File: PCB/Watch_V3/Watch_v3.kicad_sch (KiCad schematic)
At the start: 29 parts, among them J1 USB_C_Receptacle_USB2.0_16P, Q1 AO3401A, SW1 SW_DPST_x2, U1 AP2112K-3.3, U2 AP2112K-3.3, U3 AP2112K-3.3, U4 AP2112K-3.3

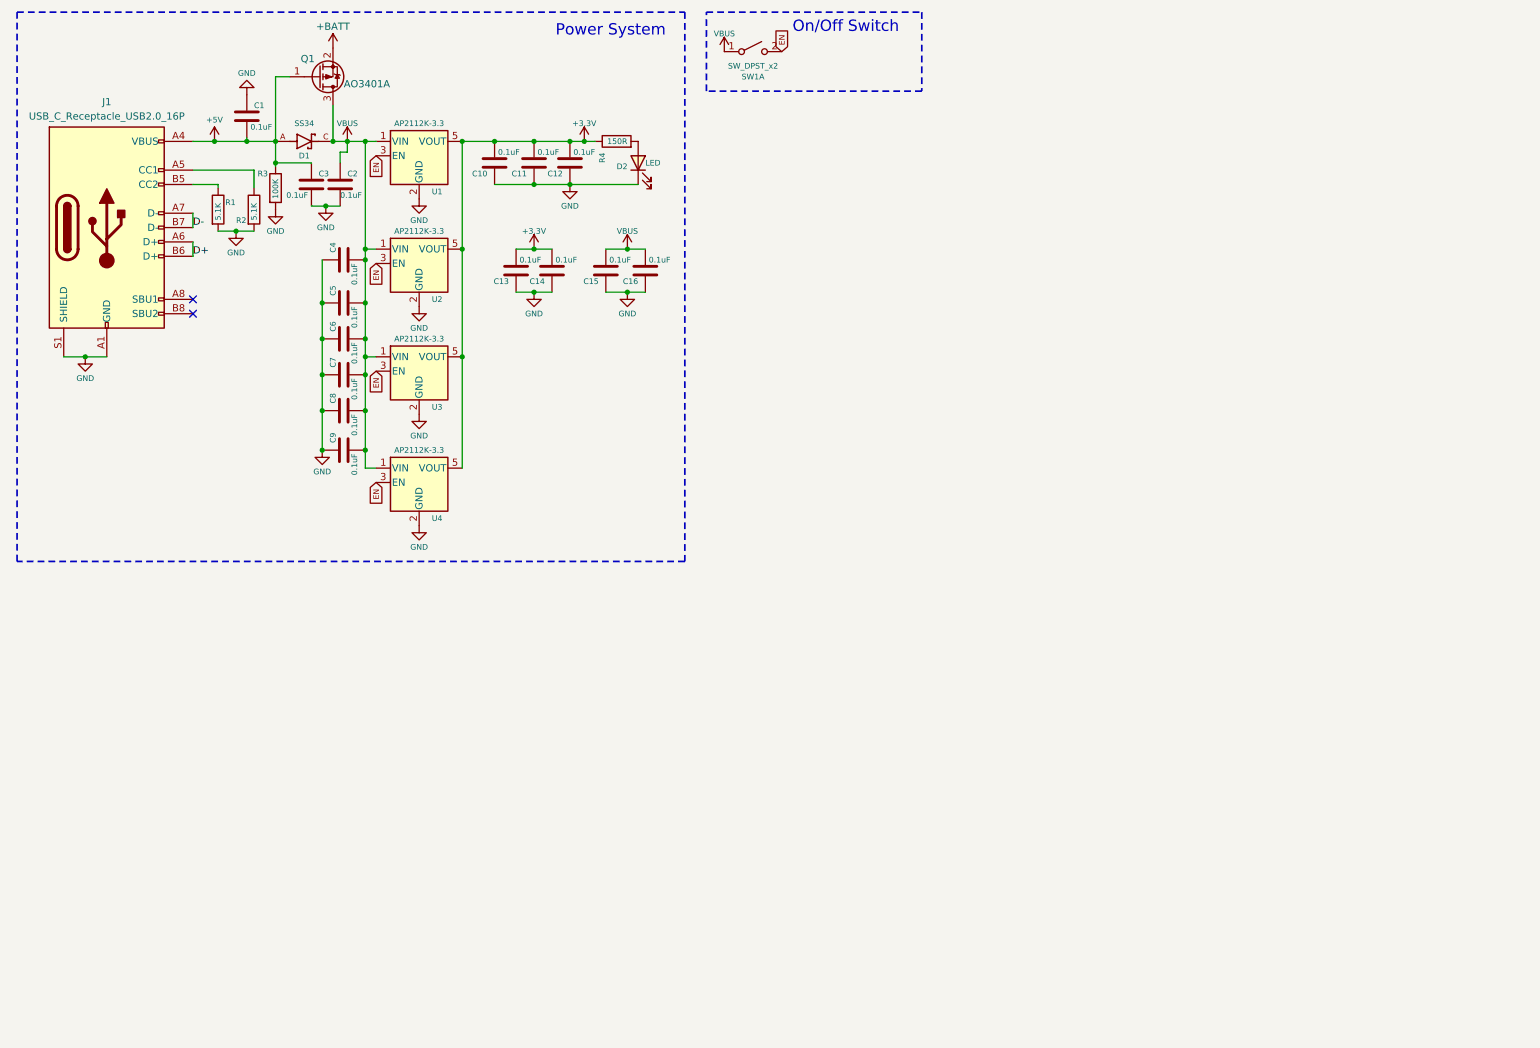
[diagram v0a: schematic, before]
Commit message: update PCB_watchV3
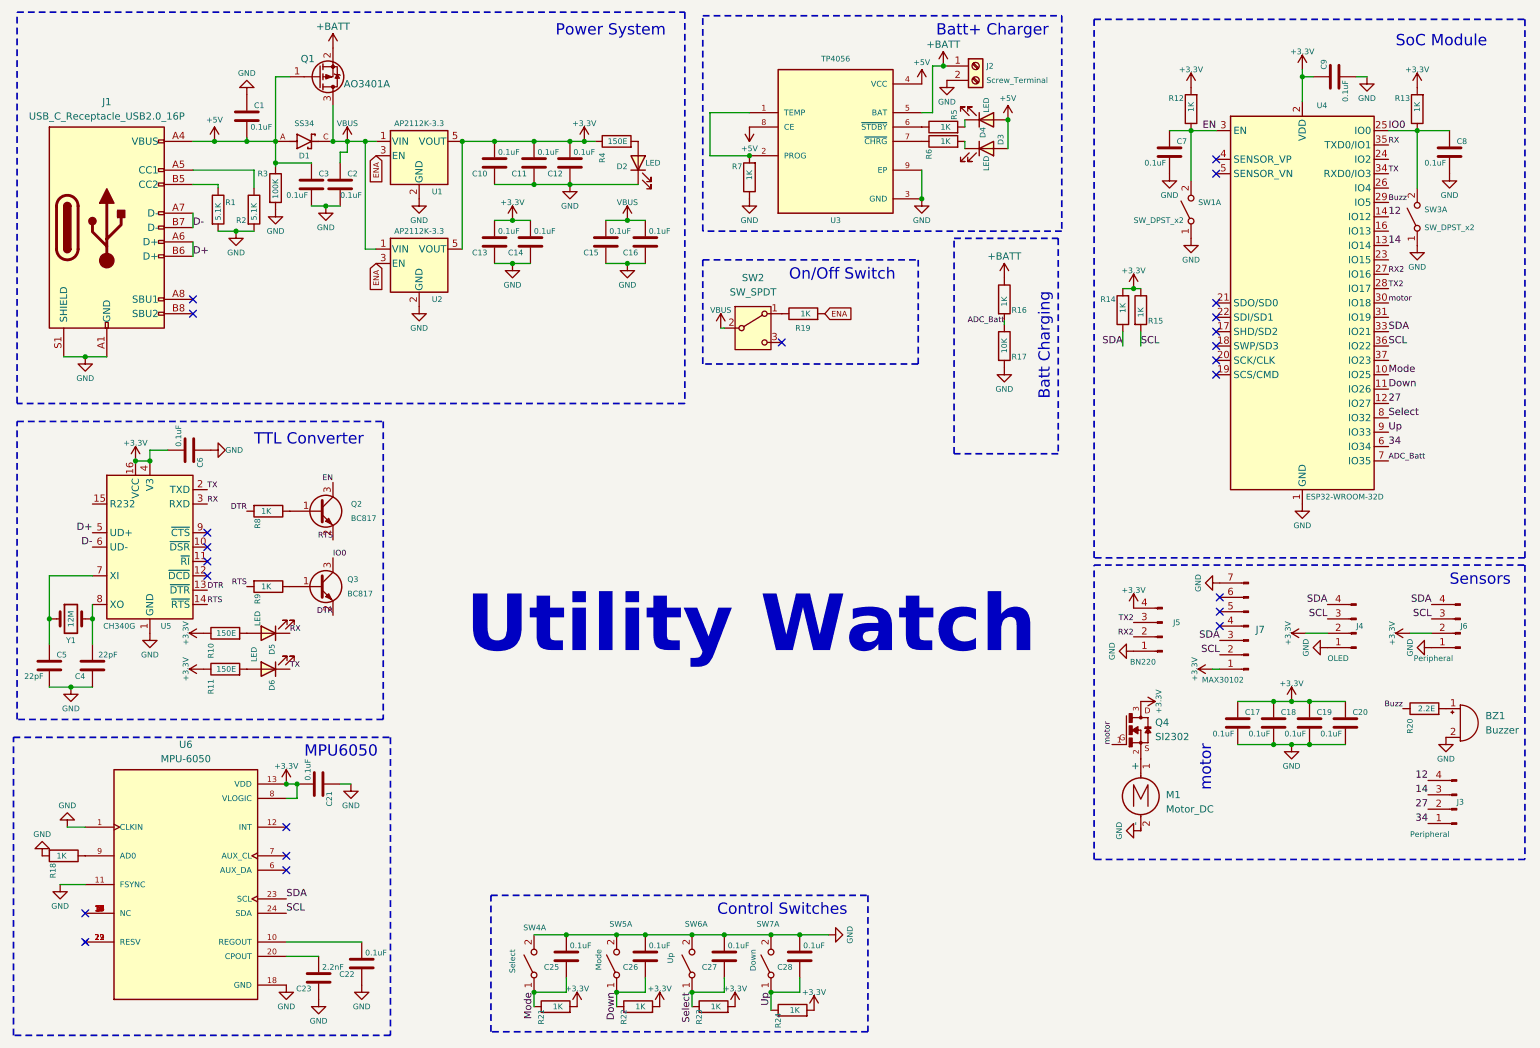
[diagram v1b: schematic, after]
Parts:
- removed U3, U4: AP2112K-3.3, Package_TO_SOT_SMD:SOT-23-5, symbol Regulator_Linear:AP2112K-3.3
- added BZ1: Buzzer, Buzzer_Beeper:Buzzer_12x9.5RM7.6, symbol Device:Buzzer
- added C17, C18, C19, C20, C21, C22, C25, C26, C27, C28: 0.1uF, Capacitor_SMD:C_0402_1005Metric, symbol Device:C
- added C23: 2.2nF, Capacitor_SMD:C_0402_1005Metric, symbol Device:C
- added D3, D4, D5, D6: LED, LED_SMD:LED_0402_1005Metric, symbol Device:LED
- added J2: Screw_Terminal, Button_Switch_SMD:solder_pad_batt, symbol Connector:Screw_Terminal_01x02
- added J3, J6: Peripheral, Button_Switch_SMD:solder_pad_4, symbol Connector:Conn_01x04_Pin
- added J4: OLED, Connector_PinHeader_2.54mm:PinHeader_1x04_P2.54mm_Vertical, symbol Connector:Conn_01x04_Pin
- added J5: BN220, Button_Switch_SMD:solder_pad_4, symbol Connector:Conn_01x04_Pin
- added J7: MAX30102, Connector_PinHeader_2.54mm:PinHeader_1x07_P2.54mm_Vertical, symbol Connector:Conn_01x07_Pin
- added M1: Motor_DC, Button_Switch_SMD:solder_motor, symbol Motor:Motor_DC
- added Q2, Q3: BC817, Package_TO_SOT_SMD:SOT-23, symbol Transistor_BJT:BC817
- added Q4: SI2302, SI2302:SOT23, symbol SI2302:SI2302
- added R10, R11: 150E, Resistor_SMD:R_01005_0402Metric, symbol Device:R
- added R12, R13, R14, R15, R16, R18, R19, R21, R22, R23, R24, R5, R6, R7, R8, R9: 1K, Resistor_SMD:R_01005_0402Metric, symbol Device:R
- added R17: 10K, Resistor_SMD:R_01005_0402Metric, symbol Device:R
- added R20: 2.2E, Resistor_SMD:R_01005_0402Metric, symbol Device:R
- added SW2: SW_SPDT, Button_Switch_THT:SW_Slide_1P2T_CK_OS102011MS2Q, symbol Switch:SW_SPDT
- added SW3: SW_DPST_x2, Button_Switch_SMD:SW_Push_1P1T_NO_6x6mm_H9.5mm, symbol Switch:SW_DPST_x2
- added SW4: Select, Button_Switch_SMD:SW_Push_1P1T_NO_6x6mm_H9.5mm, symbol Switch:SW_DPST_x2
- added SW5: Mode, Button_Switch_SMD:SW_Push_1P1T_NO_6x6mm_H9.5mm, symbol Switch:SW_DPST_x2
- added SW6: Up, Button_Switch_SMD:SW_Push_1P1T_NO_6x6mm_H9.5mm, symbol Switch:SW_DPST_x2
- added SW7: Down, Button_Switch_SMD:SW_Push_1P1T_NO_6x6mm_H9.5mm, symbol Switch:SW_DPST_x2
- added U3: TP4056, TP4056:SOP127P600X175-9N, symbol Amplifier_Audio:TP4056
- added U4: ESP32-WROOM-32D, RF_Module:ESP32-WROOM-32D, symbol RF_Module:ESP32-WROOM-32D
- added U5: CH340G, Package_SO:SOIC-16_3.9x9.9mm_P1.27mm, symbol Interface_USB:CH340G
- added U6: MPU-6050, Button_Switch_SMD:QFN50P400X400X95-24N, symbol MPU-6050:MPU-6050
- added Y1: 12M, Crystal:Crystal_HC49-4H_Vertical, symbol Device:Crystal
- C1, C10, C11, C12, C13, C14, C15, C16, C2, C3, C6, C7, C8, C9: footprint (none) -> Capacitor_SMD:C_0402_1005Metric
- C4, C5: value 0.1uF -> 22pF; footprint (none) -> Capacitor_SMD:C_0402_1005Metric
- D1: footprint SS34:DIOM7959X265N -> Capacitor_SMD:ss34_DO
- D2: footprint (none) -> LED_SMD:LED_0402_1005Metric
- J1: footprint (none) -> Connector_USB:USB_C_Receptacle_HCTL_HC-TYPE-C-16P-01A
- R1, R2, R3: footprint (none) -> Resistor_SMD:R_01005_0402Metric
- R4: value 150R -> 150E; footprint (none) -> Resistor_SMD:R_01005_0402Metric
- SW1: footprint (none) -> Button_Switch_SMD:SW_Push_1P1T_NO_6x6mm_H9.5mm
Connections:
- net +3.3V: now also C6.1, C9.2, C17.2, C18.2, C19.2, C20.2, C21.1, J4.2 (Pin_2), J5.4 (Pin_4), J6.2 (Pin_2), J7.1 (Pin_1), Q4.3, R10.1, R11.1, R12.2, R13.2, R14.2, R15.1, R21.2, R22.2, R23.2, R24.2, U4.2 (VDD), U5.16 (VCC), U5.4 (V3), U6.13 (VDD), U6.8 (VLOGIC)
- net +5V: now also D3.2 (A), D4.2 (A), U3.4 (VCC), U3.8 (CE)
- net +BATT: now also J2.1 (Pin_1), R16.1, U3.5 (BAT)
- net D+: now also U5.5 (UD+)
- net D-: now also U5.6 (UD-)
- net EN: now also C7.2, Q2.3 (C), R12.1, U4.3 (EN); no longer U1.3 (EN), U2.3 (EN)
- net GND: now also C5.1, C7.1, C8.1, C9.1, SW1.1 (A), BZ1.2 (-), C17.1, C18.1, C19.1, C20.1, C21.2, C22.2, C23.2, C25.1, C26.1, C27.1, C28.1, J2.2 (Pin_2), J4.1 (Pin_1), J5.1 (Pin_1), J6.1 (Pin_1), J7.7 (Pin_7), M1.2 (-), R17.2, R18.2, R7.1, SW3.1 (A), SW4.2 (B), SW5.2 (B), SW6.2 (B), SW7.2 (B), U3.3 (GND), U3.9 (EP), U4.1 (GND), U4.15 (GND), U4.38 (GND), U4.39 (GND), U5.1 (GND), U6.1 (CLKIN), U6.11 (FSYNC), U6.18 (GND); no longer C5.2, C7.2, C8.2, C9.2
- net VBUS: now also SW2.2 (B); no longer C4.1, C5.1, C6.1, C7.1, C8.1, C9.1, SW1.1 (A)
- new net: R7.2, U3.1 (TEMP), U3.2 (PROG)
- new net: R5.1, U3.6 (~{STDBY})
- new net: R6.1, U3.7 (~{CHRG})
- new net: Q3.1 (B), R9.1
- new net: D6.2 (A), R11.2
- new net: R19.1, SW2.1 (A)
- new net: M1.1 (+), Q4.2
- new net: D4.1 (K), R6.2
- new net: C5.2, U5.7 (XI), Y1.1
- new net: R18.1, U6.9 (AD0)
- new net: C4.1, U5.8 (XO), Y1.2
- new net: Q2.1 (B), R8.1
- new net: BZ1.1 (+), R20.2
- new net: D3.1 (K), R5.2
- new net: D5.2 (A), R10.2
- new net: C23.1, U6.20 (CPOUT)
- new net: C22.1, U6.10 (REGOUT)
- new net: U6.14 (NC), U6.15 (NC), U6.16 (NC), U6.17 (NC), U6.2 (NC), U6.3 (NC), U6.4 (NC), U6.5 (NC)
- new net: U6.19 (RESV), U6.21 (RESV), U6.22 (RESV)
- new net 12: J3.4 (Pin_4), U4.14 (IO12)
- new net 14: J3.3 (Pin_3), U4.13 (IO14)
- new net 27: J3.2 (Pin_2), U4.12 (IO27)
- new net 34: J3.1 (Pin_1), U4.6 (IO34)
- new net ADC_Batt: R16.2, R17.1, U4.7 (IO35)
- new net Buzz: R20.1, U4.29 (IO5)
- new net DTR: Q3.2 (E), R8.2, U5.13 (~{DTR})
- new net Down: C26.2, R22.1, SW5.1 (A), U4.11 (IO26)
- new net ENA: R19.2, U1.3 (EN), U2.3 (EN)
- new net IO0: C8.2, Q3.3 (C), R13.1, SW3.2 (B), U4.25 (IO0)
- new net Mode: C25.2, R21.1, SW4.1 (A), U4.10 (IO25)
- new net RTS: Q2.2 (E), R9.2, U5.14 (~{RTS})
- new net RX: D5.1 (K), U4.35 (TXD0/IO1), U5.3 (RXD)
- new net RX2: J5.2 (Pin_2), U4.27 (IO16)
- new net SCL: J4.3 (Pin_3), J6.3 (Pin_3), J7.2 (Pin_2), R15.2, U4.36 (IO22), U6.24 (SDA)
- new net SDA: J4.4 (Pin_4), J6.4 (Pin_4), J7.3 (Pin_3), R14.1, U4.33 (IO21), U6.23 (SCL)
- new net Select: C27.2, R23.1, SW6.1 (A), U4.8 (IO32)
- new net TX: D6.1 (K), U4.34 (RXD0/IO3), U5.2 (TXD)
- new net TX2: J5.3 (Pin_3), U4.28 (IO17)
- new net Up: C28.2, R24.1, SW7.1 (A), U4.9 (IO33)
- new net motor: Q4.1, U4.30 (IO18)
- no-connect marks 2 -> 23
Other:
- note added: "Batt Charging"
- note added: "Batt+ Charger"
- note added: "Control Switches"
- note added: "MPU6050"
- note added: "Sensors"
- note added: "SoC Module"
- note added: "TTL Converter"
- note added: "Utility Watch"
- note added: "motor"
- moved on the sheet: C13, C14, C15, C16
